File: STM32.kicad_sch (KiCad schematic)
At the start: 5 parts, among them SW1 SW_Push, U1 STM32F091RCTx

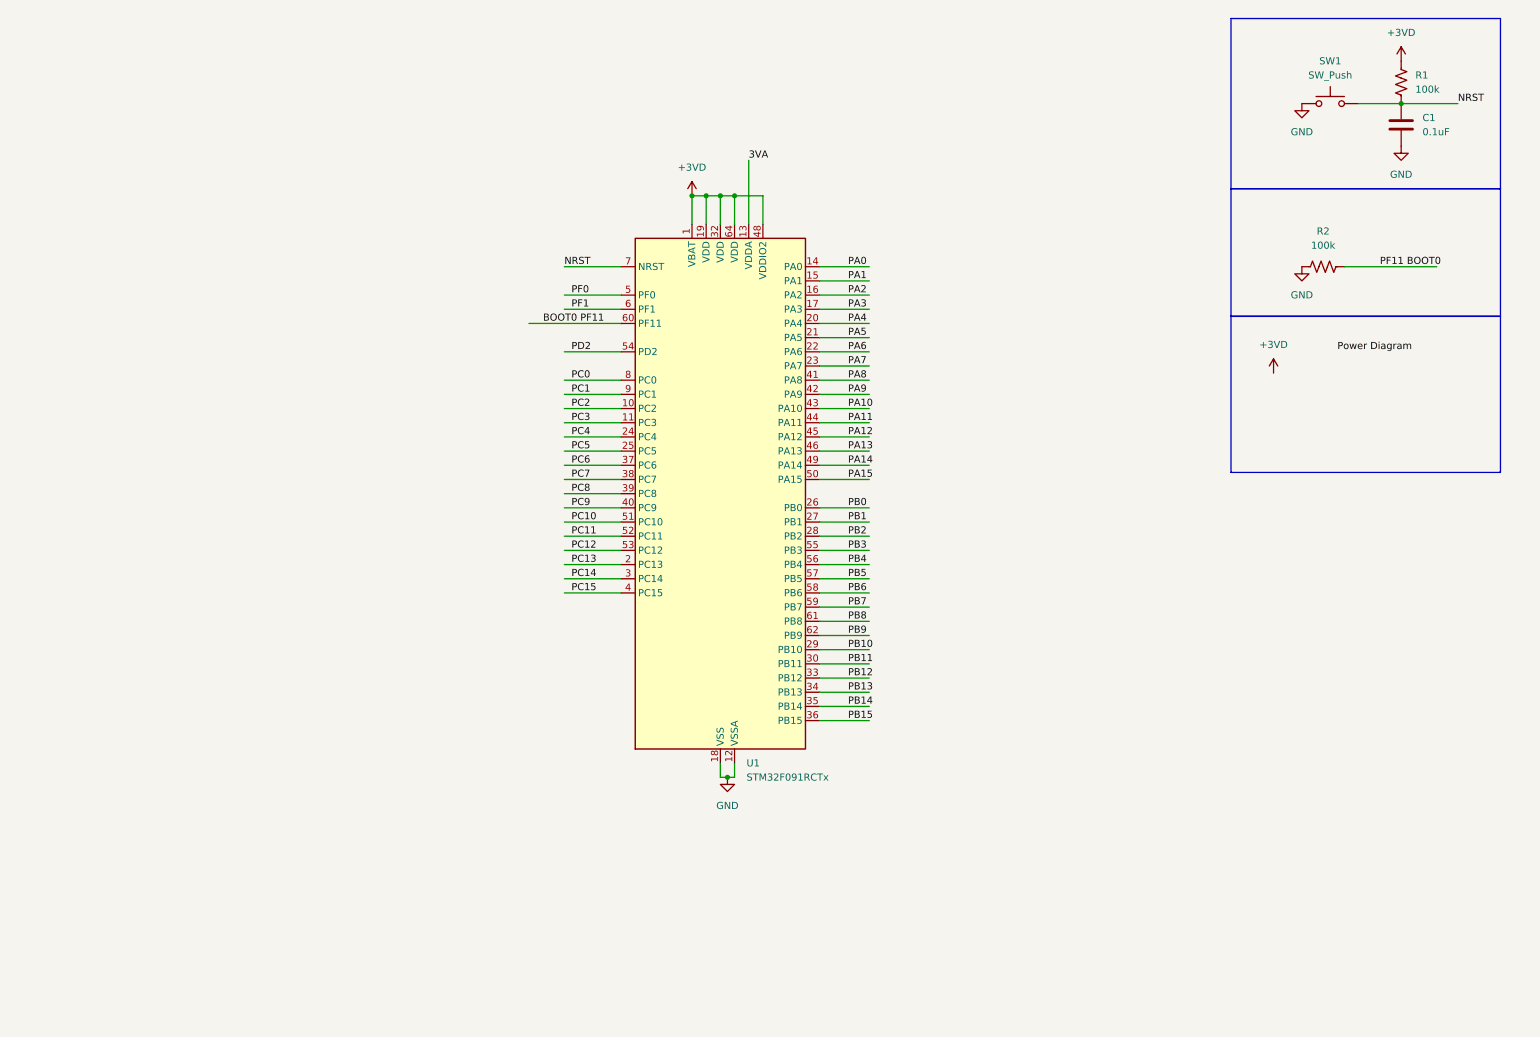
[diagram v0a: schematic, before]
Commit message: Add files via upload
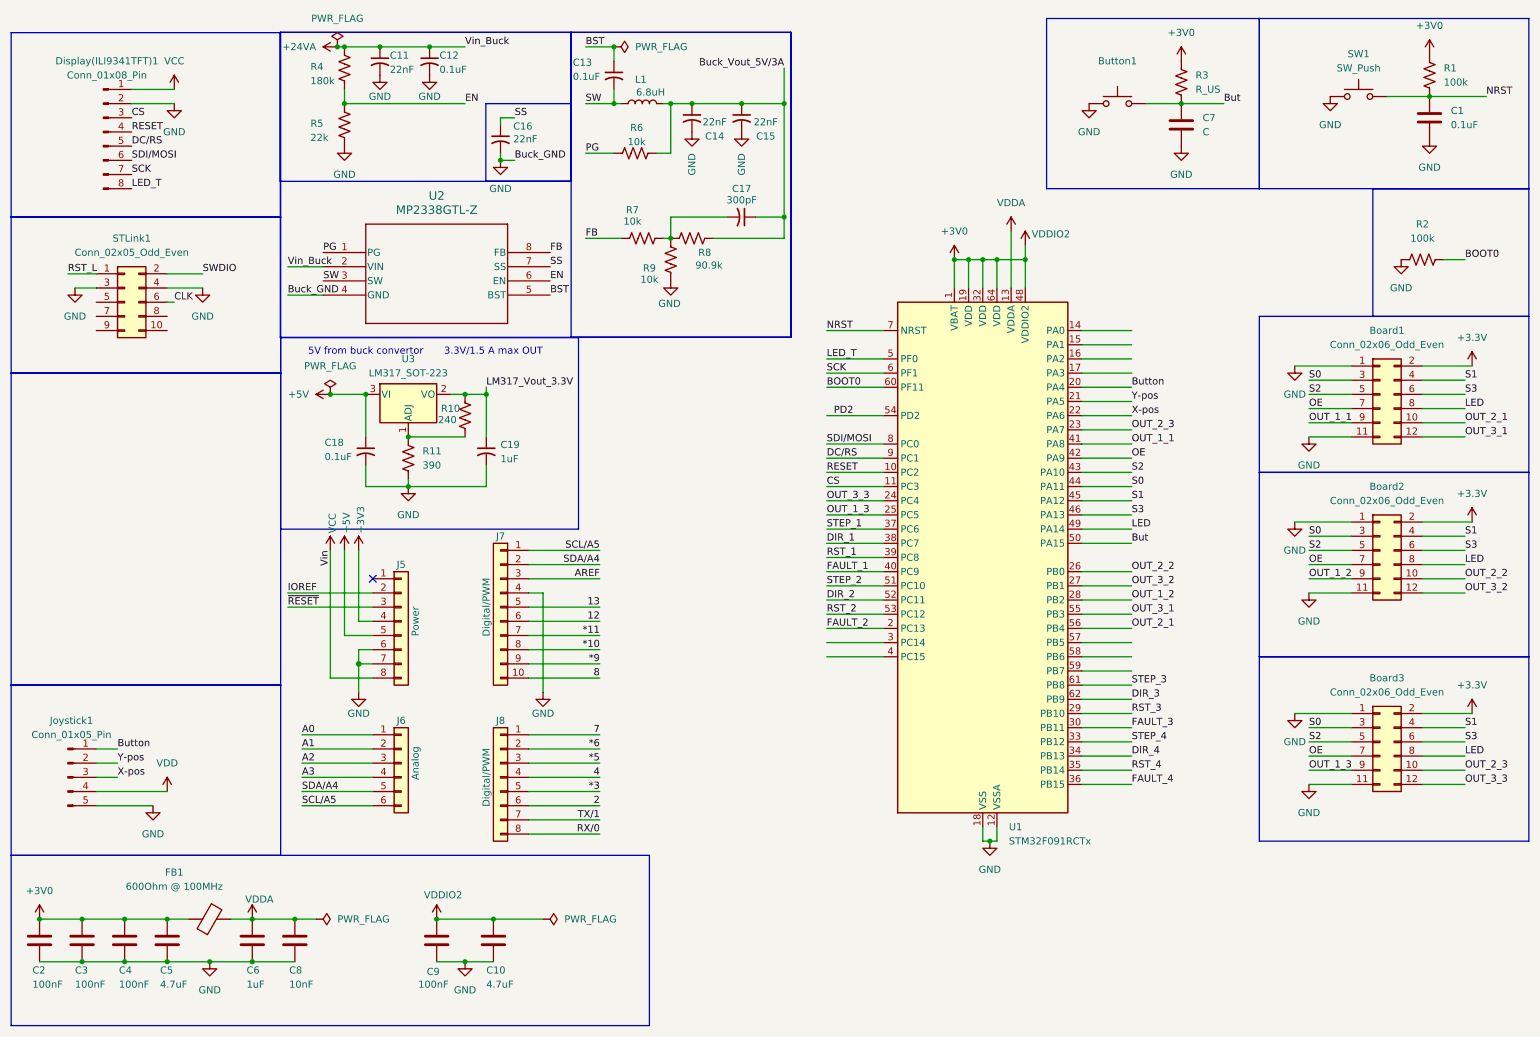
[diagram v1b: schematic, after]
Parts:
- added Board1, Board2, Board3: Conn_02x06_Odd_Even, Connector_PinHeader_1.00mm:PinHeader_2x06_P1.00mm_Vertical, symbol Connector_Generic:Conn_02x06_Odd_Even
- added Button1: ~, Button_Switch_SMD:SW_SPST_TL3342, symbol Switch:SW_Push
- added C10, C5: 4.7uF, Capacitor_SMD:C_0603_1608Metric, symbol Device:C
- added C11, C14, C15, C16: 22nF, Capacitor_SMD:C_0805_2012Metric, symbol Device:C_Small_US
- added C12, C13, C18: 0.1uF, Capacitor_SMD:C_0805_2012Metric, symbol Device:C_Small_US
- added C17: 300pF, Capacitor_SMD:C_0805_2012Metric, symbol Device:C_Small_US
- added C19: 1uF, Capacitor_SMD:C_0805_2012Metric, symbol Device:C_Small_US
- added C2, C3, C4, C9: 100nF, Capacitor_SMD:C_0603_1608Metric, symbol Device:C
- added C6: 1uF, Capacitor_SMD:C_0603_1608Metric, symbol Device:C
- added C7: C, Capacitor_SMD:C_0603_1608Metric, symbol Device:C
- added C8: 10nF, Capacitor_SMD:C_0603_1608Metric, symbol Device:C
- added Display(ILI9341TFT)1: Conn_01x08_Pin, Connector_PinHeader_1.00mm:PinHeader_1x08_P1.00mm_Vertical, symbol Connector:Conn_01x08_Pin
- added FB1: 600Ohm @ 100MHz, Resistor_SMD:R_0603_1608Metric, symbol Device:FerriteBead
- added J5: Power, Connector_PinSocket_2.54mm:PinSocket_1x08_P2.54mm_Vertical, symbol Connector_Generic:Conn_01x08
- added J6: Analog, Connector_PinSocket_2.54mm:PinSocket_1x06_P2.54mm_Vertical, symbol Connector_Generic:Conn_01x06
- added J7: Digital/PWM, Connector_PinSocket_2.54mm:PinSocket_1x10_P2.54mm_Vertical, symbol Connector_Generic:Conn_01x10
- added J8: Digital/PWM, Connector_PinSocket_2.54mm:PinSocket_1x08_P2.54mm_Vertical, symbol Connector_Generic:Conn_01x08
- added Joystick1: Conn_01x05_Pin, Connector_PinHeader_1.00mm:PinHeader_1x05_P1.00mm_Vertical, symbol Connector:Conn_01x05_Pin
- added L1: 6.8uH, Inductor_SMD:L_0805_2012Metric, symbol Device:L
- added R10: 240, Resistor_SMD:R_0805_2012Metric, symbol Device:R_US
- added R11: 390, Resistor_SMD:R_0805_2012Metric, symbol Device:R_US
- added R3: R_US, Resistor_SMD:R_0603_1608Metric, symbol Device:R_US
- added R4: 180k, Resistor_SMD:R_0805_2012Metric, symbol Device:R_US
- added R5: 22k, Resistor_SMD:R_0805_2012Metric, symbol Device:R_US
- added R6, R7, R9: 10k, Resistor_SMD:R_0805_2012Metric, symbol Device:R_US
- added R8: 90.9k, Resistor_SMD:R_0805_2012Metric, symbol Device:R_US
- added STLink1: Conn_02x05_Odd_Even, Connector_PinHeader_1.00mm:PinHeader_2x05_P1.00mm_Vertical, symbol Connector_Generic:Conn_02x05_Odd_Even
- added U2: MP2338GTL-Z, footprints:SOT583_MP2338_MNP, symbol Power Convertor:MP2338GTL-Z
- added U3: LM317_SOT-223, Package_TO_SOT_SMD:SOT-223-3_TabPin2, symbol Regulator_Linear:LM317_SOT-223
- C1: footprint (none) -> Capacitor_SMD:C_0603_1608Metric
- R1, R2: footprint (none) -> Resistor_SMD:R_0603_1608Metric
- SW1: footprint (none) -> Button_Switch_SMD:SW_SPST_TL3342
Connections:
- net PF11 BOOT0 is gone; now on net BOOT0: R2.2
- net GND: now also Board1.1 (Pin_1), Board1.11 (Pin_11), Board2.1 (Pin_1), Board2.11 (Pin_11), Board3.1 (Pin_1), Board3.11 (Pin_11), Button1.1, C10.2, C11.2, C12.2, C14.2, C15.2, C16.2, C18.2, C19.2, C2.2, C3.2, C4.2, C5.2, C6.2, C7.2, C8.2, C9.2, Display(ILI9341TFT)1.2 (Pin_2), J5.6 (Pin_6), J5.7 (Pin_7), J7.4 (Pin_4), Joystick1.5 (Pin_5), R11.2, R5.2, R9.2, STLink1.3 (Pin_3), STLink1.4 (Pin_4), U2.4 (GND)
- net +3VD renamed +3V0
- net +3V0: now also C10.1, C2.1, C3.1, C4.1, C5.1, C9.1, FB1.1, R3.1
- net 3VA renamed VDDA
- net VDDA: now also C6.1, C8.1, FB1.2
- net BOOT0 PF11 renamed BOOT0
- net PA0: no longer names the net of U1.14 (PA0)
- net PA1: no longer names the net of U1.15 (PA1)
- net PA10 renamed S2
- net S2: now also Board1.5 (Pin_5), Board2.5 (Pin_5), Board3.5 (Pin_5)
- net PA11 renamed S0
- net S0: now also Board1.3 (Pin_3), Board2.3 (Pin_3), Board3.3 (Pin_3)
- net PA12 renamed S1
- net S1: now also Board1.4 (Pin_4), Board2.4 (Pin_4), Board3.4 (Pin_4)
- net PA13 renamed S3
- net S3: now also Board1.6 (Pin_6), Board2.6 (Pin_6), Board3.6 (Pin_6)
- net PA14 renamed LED
- net LED: now also Board1.8 (Pin_8), Board2.8 (Pin_8), Board3.8 (Pin_8)
- net PA15 renamed But
- net But: now also Button1.2, C7.1, R3.2
- net PA2: no longer names the net of U1.16 (PA2)
- net PA3: no longer names the net of U1.17 (PA3)
- net PA4 renamed Button
- net Button: now also Joystick1.1 (Pin_1)
- net PA5 renamed Y-pos
- net Y-pos: now also Joystick1.2 (Pin_2)
- net PA6 renamed X-pos
- net X-pos: now also Joystick1.3 (Pin_3)
- net PA7 renamed OUT_2_3
- net OUT_2_3: now also Board3.10 (Pin_10)
- net PA8 renamed OUT_1_1
- net OUT_1_1: now also Board1.9 (Pin_9)
- net PA9 renamed OE
- net OE: now also Board1.7 (Pin_7), Board2.7 (Pin_7), Board3.7 (Pin_7)
- net PB0 renamed OUT_2_2
- net OUT_2_2: now also Board2.10 (Pin_10)
- net PB1 renamed OUT_3_2
- net OUT_3_2: now also Board2.12 (Pin_12)
- net PB10 renamed RST_3
- net PB11 renamed FAULT_3
- net PB12 renamed STEP_4
- net PB13 renamed DIR_4
- net PB14 renamed RST_4
- net PB15 renamed FAULT_4
- net PB2 renamed OUT_1_2
- net OUT_1_2: now also Board2.9 (Pin_9)
- net PB3 renamed OUT_3_1
- net OUT_3_1: now also Board1.12 (Pin_12)
- net PB4 renamed OUT_2_1
- net OUT_2_1: now also Board1.10 (Pin_10)
- net PB5: no longer names the net of U1.57 (PB5)
- net PB6: no longer names the net of U1.58 (PB6)
- net PB7: no longer names the net of U1.59 (PB7)
- net PB8 renamed STEP_3
- net PB9 renamed DIR_3
- net PC0 renamed SDI/MOSI
- net SDI/MOSI: now also Display(ILI9341TFT)1.6 (Pin_6)
- net PC1 renamed DC/RS
- net DC/RS: now also Display(ILI9341TFT)1.5 (Pin_5)
- net PC10 renamed STEP_2
- net PC11 renamed DIR_2
- net PC12 renamed RST_2
- net PC13 renamed FAULT_2
- net PC14: no longer names the net of U1.3 (PC14)
- net PC15: no longer names the net of U1.4 (PC15)
- net PC2 renamed RESET
- net RESET: now also Display(ILI9341TFT)1.4 (Pin_4)
- net PC3 renamed CS
- net CS: now also Display(ILI9341TFT)1.3 (Pin_3)
- net PC4 renamed OUT_3_3
- net OUT_3_3: now also Board3.12 (Pin_12)
- net PC5 renamed OUT_1_3
- net OUT_1_3: now also Board3.9 (Pin_9)
- net PC6 renamed STEP_1
- net PC7 renamed DIR_1
- net PC8 renamed RST_1
- net PC9 renamed FAULT_1
- net PF0 renamed LED_T
- net LED_T: now also Display(ILI9341TFT)1.8 (Pin_8)
- net PF1 renamed SCK
- net SCK: now also Display(ILI9341TFT)1.7 (Pin_7)
- new net: C17.2, R7.1, R8.1, R9.1
- new net: R10.2, R11.1, U3.1 (ADJ)
- new net *10: J7.8 (Pin_8)
- new net *11: J7.7 (Pin_7)
- new net *3: J8.5 (Pin_5)
- new net *5: J8.3 (Pin_3)
- new net *6: J8.2 (Pin_2)
- new net *9: J7.9 (Pin_9)
- new net +24VA: C11.1, C12.1, R4.1, U2.2 (VIN)
- new net +3.3V: Board1.2 (Pin_2), Board2.2 (Pin_2), Board3.2 (Pin_2)
- new net +3V3: J5.4 (Pin_4)
- new net +5V: C18.1, J5.5 (Pin_5), U3.3 (VI)
- new net 12: J7.6 (Pin_6)
- new net 13: J7.5 (Pin_5)
- new net 2: J8.6 (Pin_6)
- new net 4: J8.4 (Pin_4)
- new net 7: J8.1 (Pin_1)
- new net 8: J7.10 (Pin_10)
- new net A0: J6.1 (Pin_1)
- new net A1: J6.2 (Pin_2)
- new net A2: J6.3 (Pin_3)
- new net A3: J6.4 (Pin_4)
- new net AREF: J7.3 (Pin_3)
- new net BST: C13.1, U2.5 (BST)
- new net Buck_Vout_5V/3A: C14.1, C15.1, C17.1, L1.2, R6.1, R8.2
- new net CLK: STLink1.6 (Pin_6)
- new net EN: R4.2, R5.1, U2.6 (EN)
- new net FB: R7.2, U2.8 (FB)
- new net IOREF: J5.2 (Pin_2)
- new net LM317_Vout_3.3V: C19.1, R10.1, U3.2 (VO)
- new net PG: R6.2, U2.1 (PG)
- new net RST_L: STLink1.1 (Pin_1)
- new net RX/0: J8.8 (Pin_8)
- new net SCL/A5: J6.6 (Pin_6), J7.1 (Pin_1)
- new net SDA/A4: J6.5 (Pin_5), J7.2 (Pin_2)
- new net SS: C16.1, U2.7 (SS)
- new net SW: C13.2, L1.1, U2.3 (SW)
- new net SWDIO: STLink1.2 (Pin_2)
- new net TX/1: J8.7 (Pin_7)
- new net VCC: Display(ILI9341TFT)1.1 (Pin_1), J5.8 (Pin_8)
- new net VDD: Joystick1.4 (Pin_4)
- new net ~{RESET}: J5.3 (Pin_3)
- no-connect marks 0 -> 1
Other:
- note added: "3.3V/1.5 A max OUT"
- note added: "5V from buck convertor"
- moved on the sheet: C1, R1, R2, SW1, U1
